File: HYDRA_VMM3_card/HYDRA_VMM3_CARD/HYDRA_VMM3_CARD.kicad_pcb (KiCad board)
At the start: 6 copper layers, 80 x 61 mm, 81 parts, among them J1 ME1014010101011

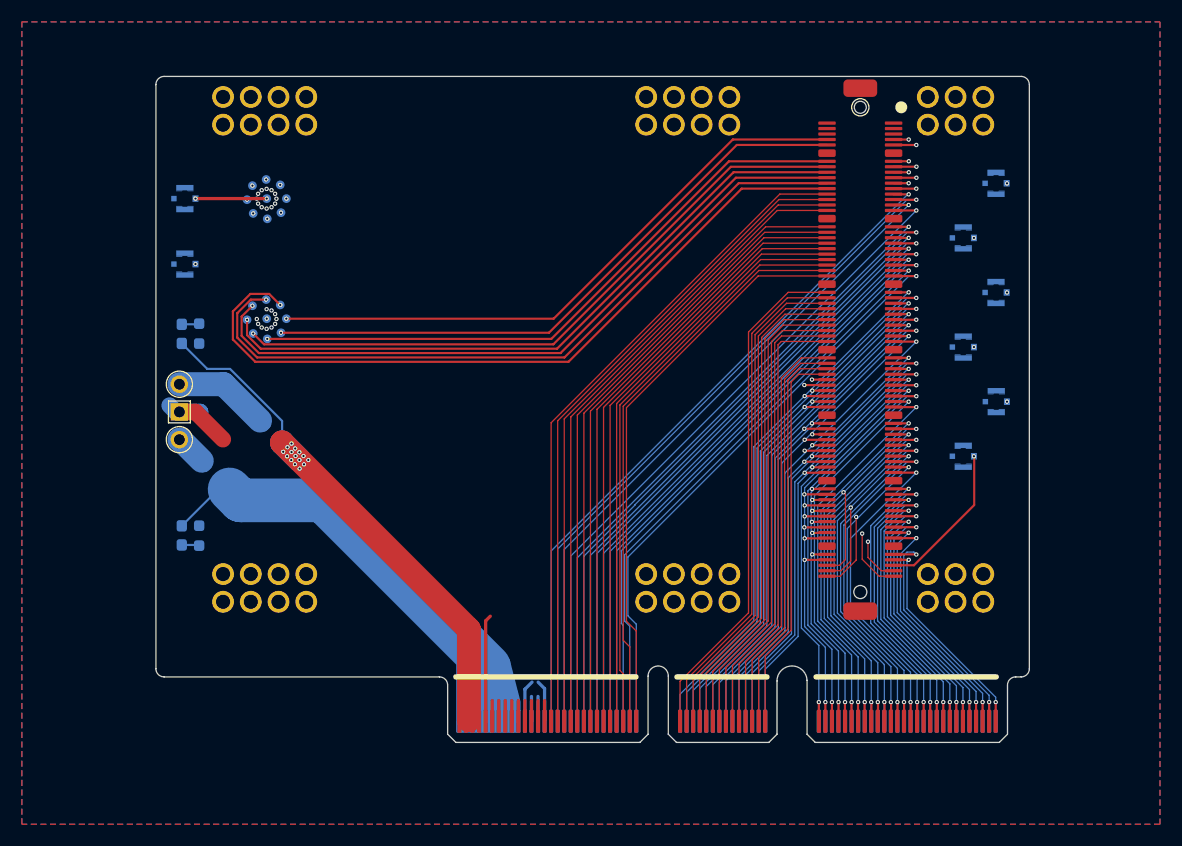
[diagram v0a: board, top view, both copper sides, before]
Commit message: .
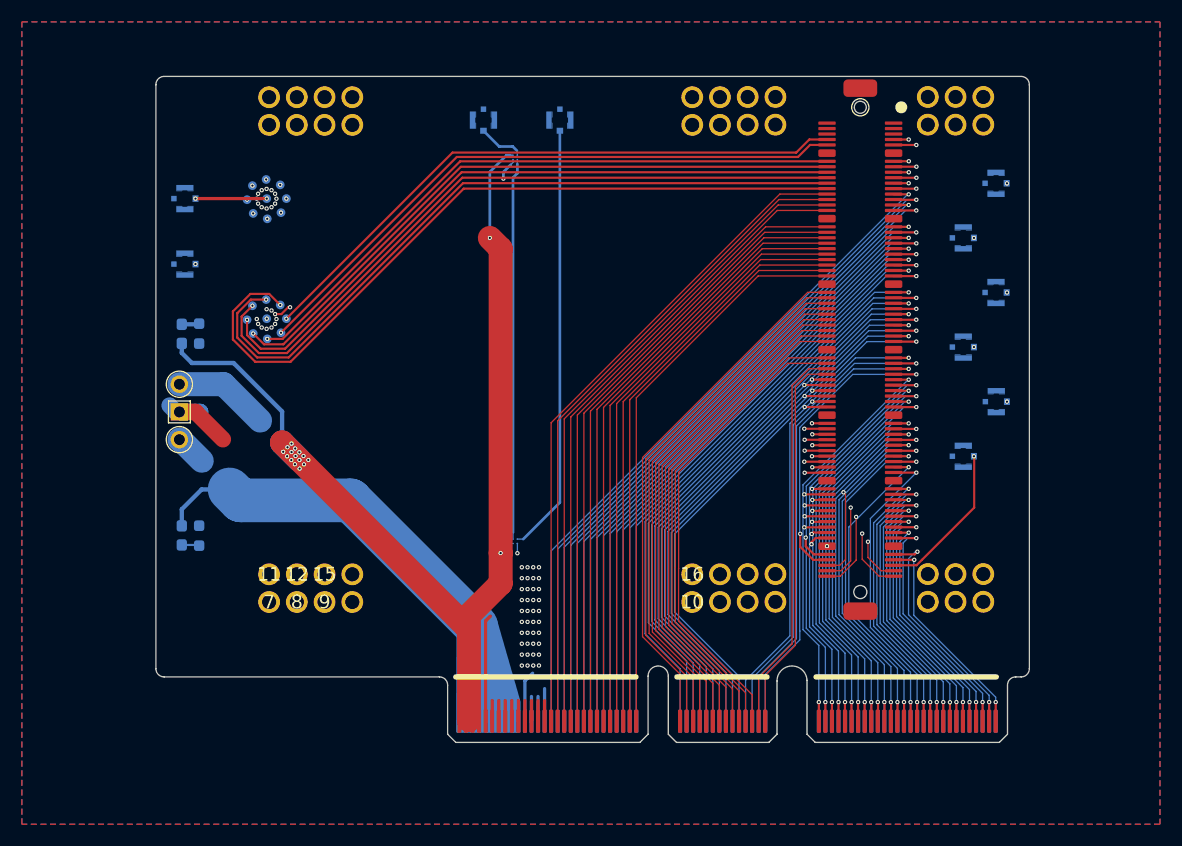
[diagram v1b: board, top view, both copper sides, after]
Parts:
- removed the ? at (73.5, 80.9)
- removed the ? at (107.2, 78.4)
- removed the ? at (107.2, 80.9)
- removed the ? at (71.0, 78.4)
- removed the ? at (73.5, 78.4)
- removed the ? at (68.5, 80.9)
- removed the ? at (71.0, 80.9)
- removed the ? at (68.5, 78.4)
- added 17: , , F.Cu at (114.0, 80.9)
- added 18: , , F.Cu at (116.5, 80.9)
- added 19: , , F.Cu at (119.0, 80.9)
- added 20: , , F.Cu at (114.0, 78.4)
- added 21: , , F.Cu at (116.5, 78.4)
- added 22: , , F.Cu at (119.0, 78.4)
- added 23: , , F.Cu at (80.3, 80.9)
- added 24: , , F.Cu at (80.3, 78.4)
- added Temp_1: ~, IPEX:TMP104, B.Cu at (95.2, 40.2)
- added Temp_2: ~, IPEX:TMP104, B.Cu at (95.2, 75.4)
- added Temp_RX1: 20449-001E-03, IPEX:IPEX_20449-001E-03, B.Cu at (99.3, 36.8)
- added Temp_TX1: 20449-001E-03, IPEX:IPEX_20449-001E-03, B.Cu at (92.3, 36.8)
- moved 11 39.6 mm to (72.7, 78.4)
- moved 12 39.6 mm to (75.2, 78.4)
- moved 8 37.1 mm to (75.2, 80.9)
- moved 7 37.1 mm to (72.7, 80.9)
- moved 9 37.1 mm to (77.7, 80.9)
- moved 16 35.4 mm to (111.4, 78.4)
- moved ? 4.22 mm to (72.7, 37.2)
- moved ? 4.22 mm to (72.7, 34.7)
- moved 1 4.22 mm to (114.0, 37.2)
- moved 13 4.22 mm to (80.3, 37.2)
- moved 14 4.22 mm to (80.3, 34.7)
- moved 4 4.22 mm to (114.0, 34.7)
- moved ? 4.22 mm to (111.4, 37.2)
- moved ? 4.22 mm to (77.7, 37.2)
- moved ? 4.22 mm to (111.4, 34.7)
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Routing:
- net P1: track 48.9 -> 97.7 mm, vias 15 -> 17
- net RX: track 0.00 -> 39.3 mm
- net Net-(Temp_1-RX): track 0.00 -> 34.9 mm
- net Ch_92: track 33.1 -> 50.7 mm
- net Ch_90: track 33.5 -> 51.1 mm
- net Ch_88: track 34.0 -> 51.6 mm
- net Ch_86: track 34.6 -> 52.0 mm
- net Ch_84: track 36.0 -> 52.9 mm
- net Ch_82: track 36.7 -> 53.4 mm
- net Ch_80: track 37.1 -> 53.8 mm
- net Ch_78: track 37.6 -> 54.3 mm
- net Ch_76: track 38.0 -> 54.7 mm
- net Ch_74: track 38.6 -> 55.2 mm
- net Ch_63: track 43.6 -> 51.1 mm
- net Ch_61: track 43.3 -> 50.1 mm
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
